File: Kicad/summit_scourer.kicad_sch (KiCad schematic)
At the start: 4 parts, among them J2 Conn_Coaxial, J7 Conn_01x06_Socket

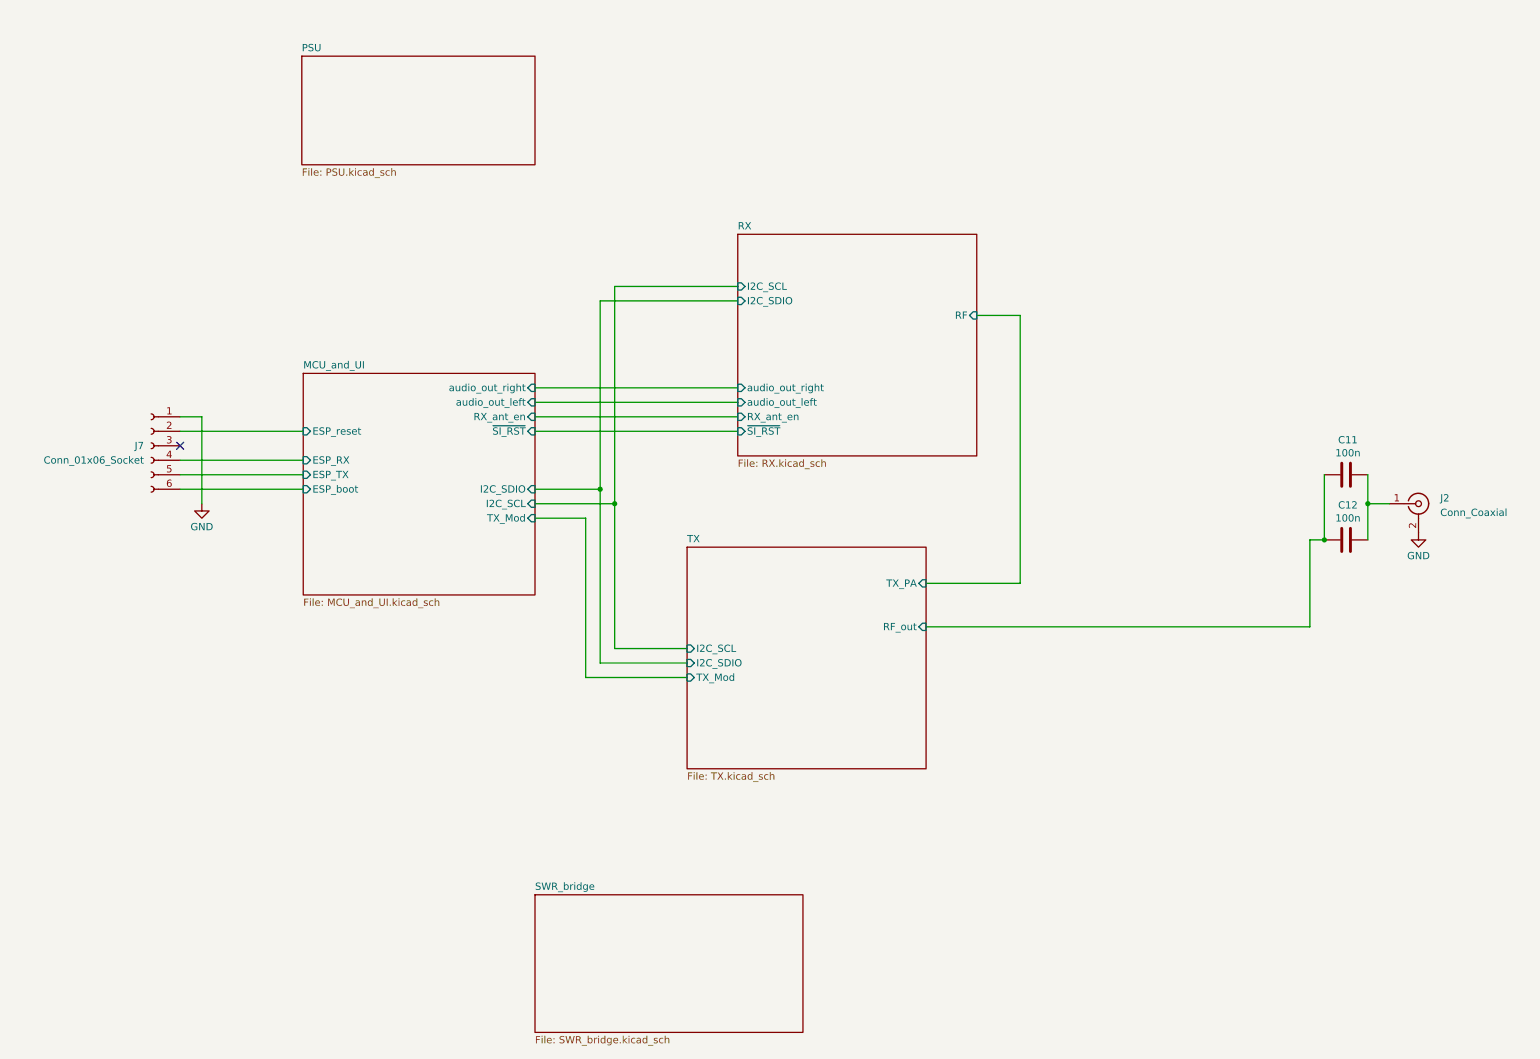
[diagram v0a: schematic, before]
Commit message: Add files via upload
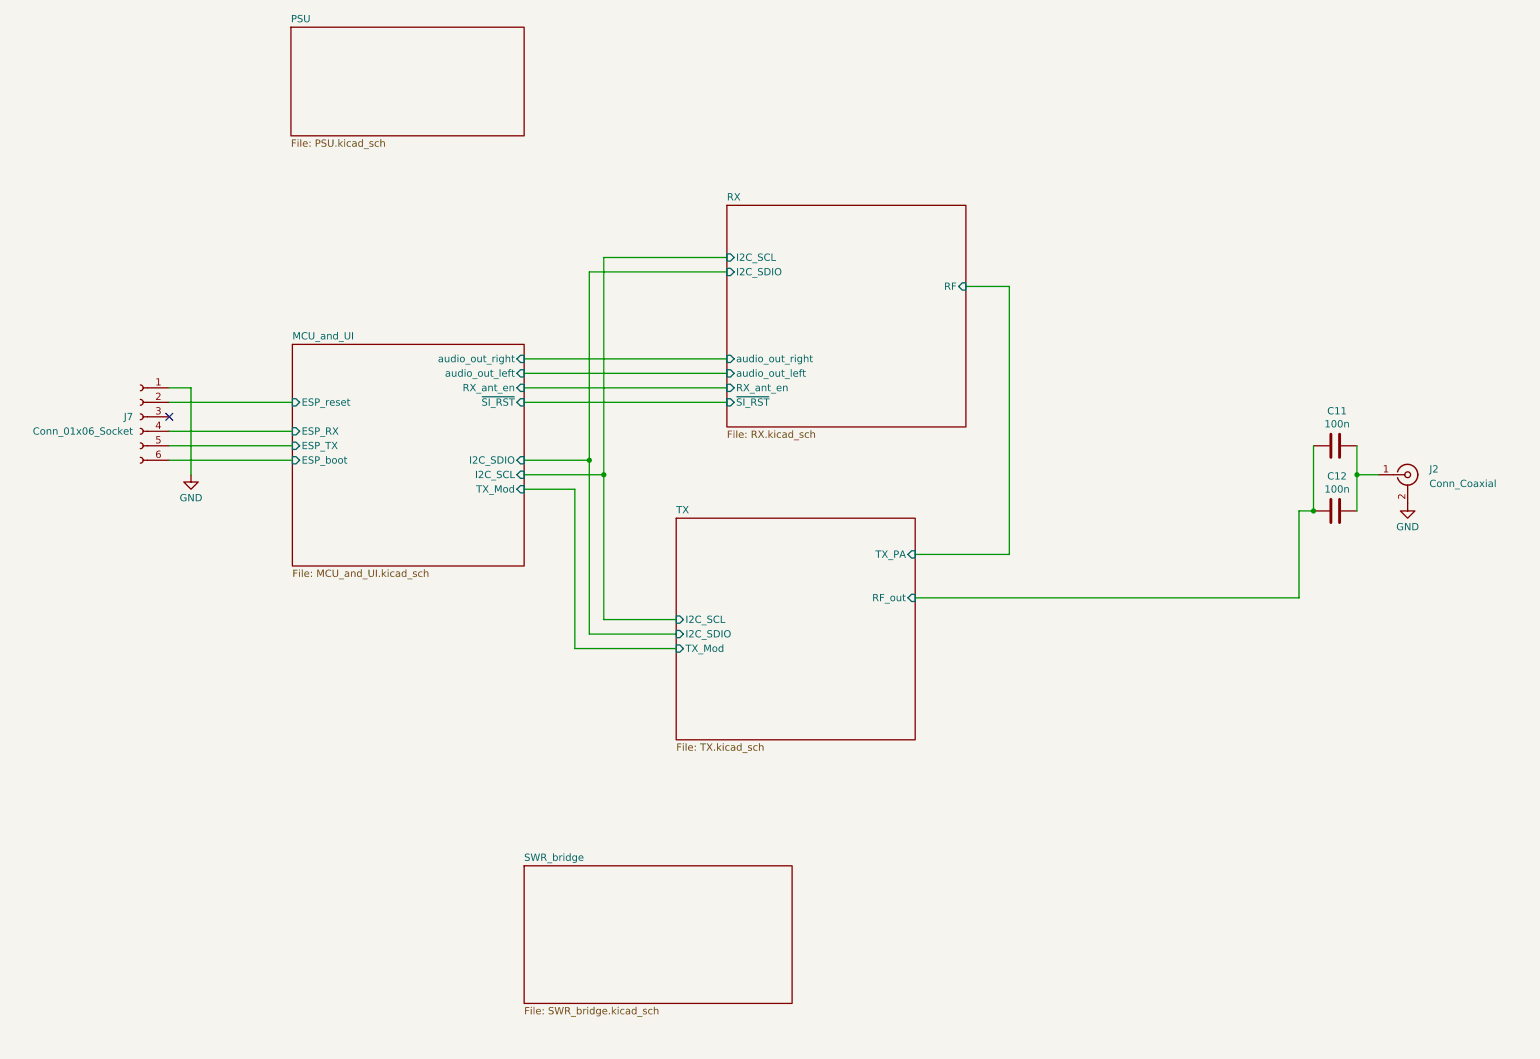
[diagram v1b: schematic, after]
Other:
- moved on the sheet: C11, C12, J2, J7
